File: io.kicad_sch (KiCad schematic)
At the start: 20 parts, among them J3 USB_C_Receptacle_USB2.0, J4 Conn_01x06_Male, U3 USBLC6-2SC6

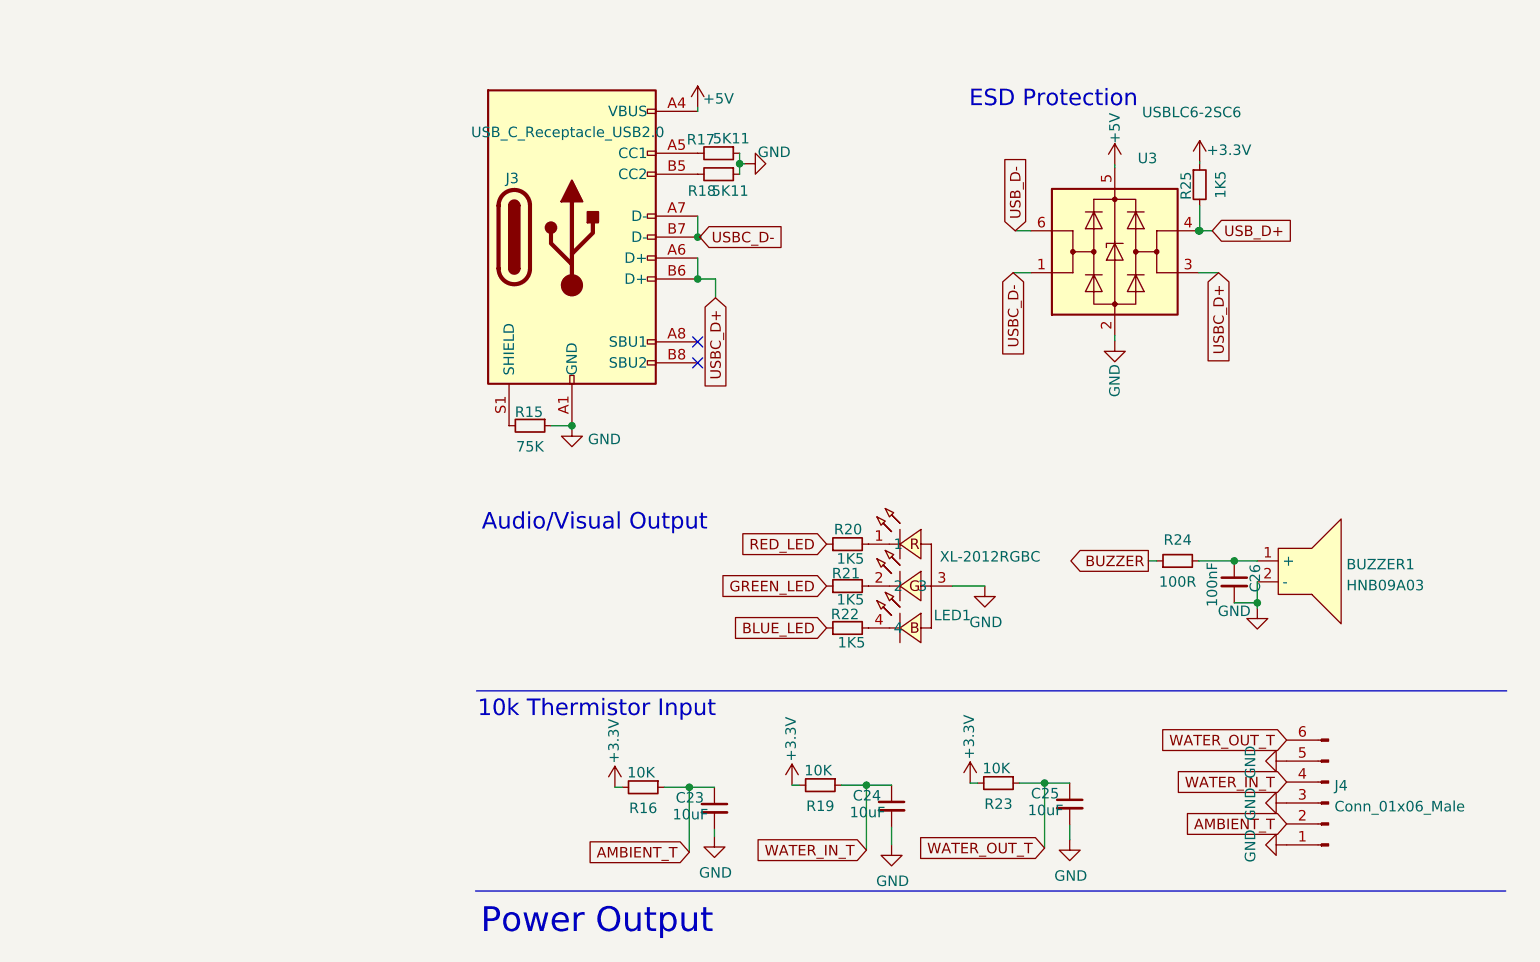
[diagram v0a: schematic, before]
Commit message: rev-7 ready
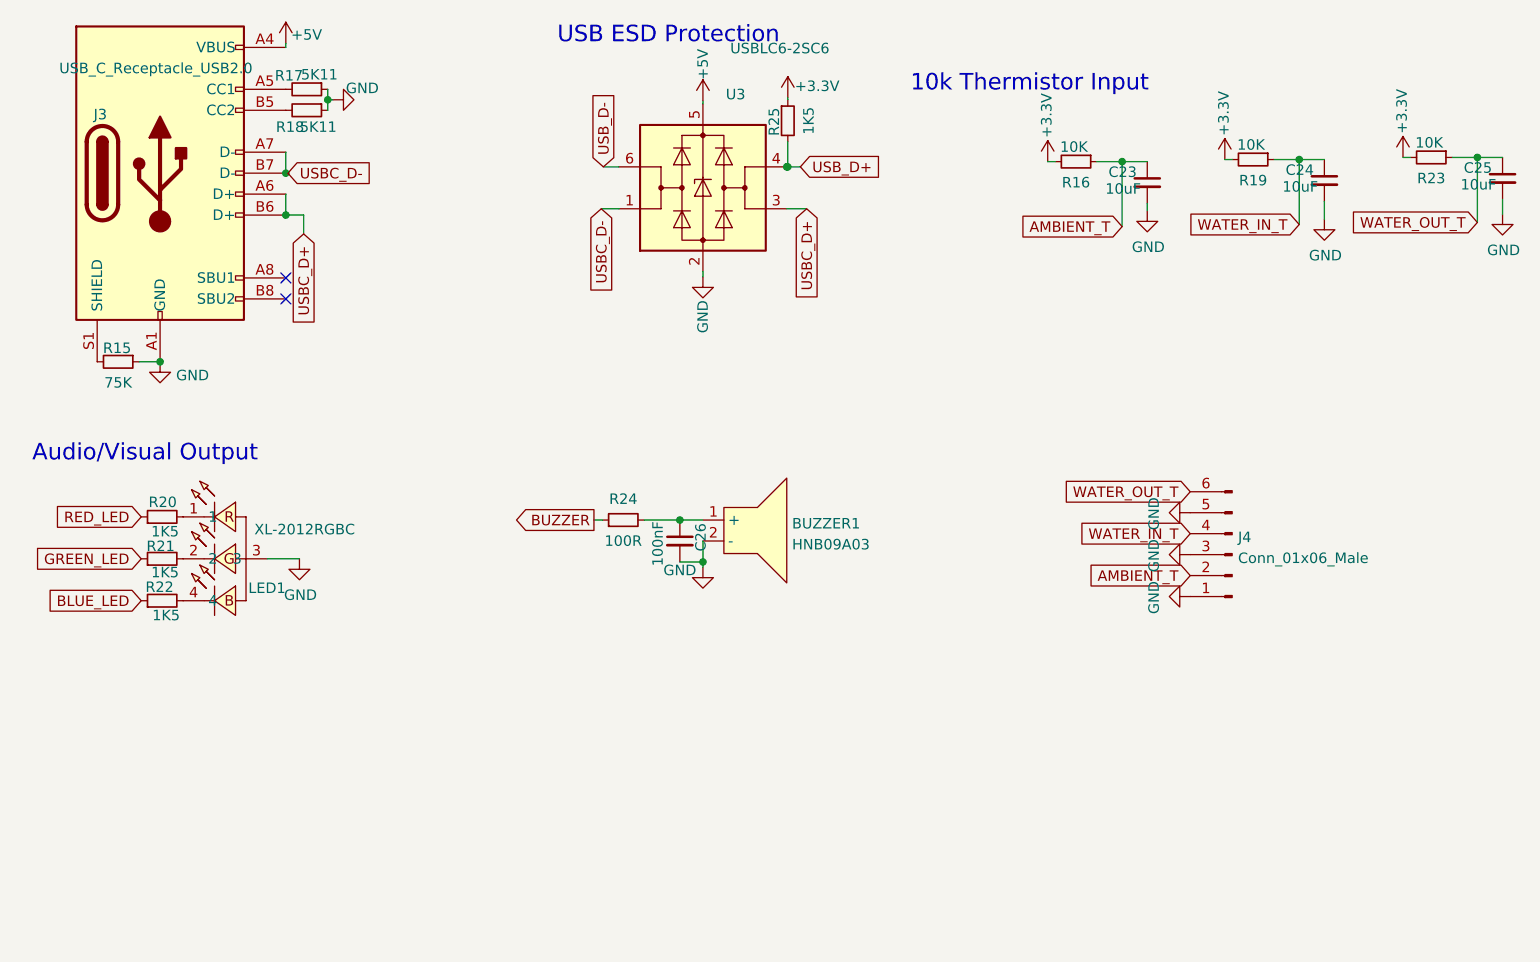
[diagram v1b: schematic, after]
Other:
- note added: "USB ESD Protection"
- note removed: "ESD Protection"
- note removed: "Power Output"
- moved on the sheet: BUZZER1, C23, C24, C25, C26, J3, J4, LED1, R15, R16, R17, R18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
